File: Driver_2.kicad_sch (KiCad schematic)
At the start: 34 parts

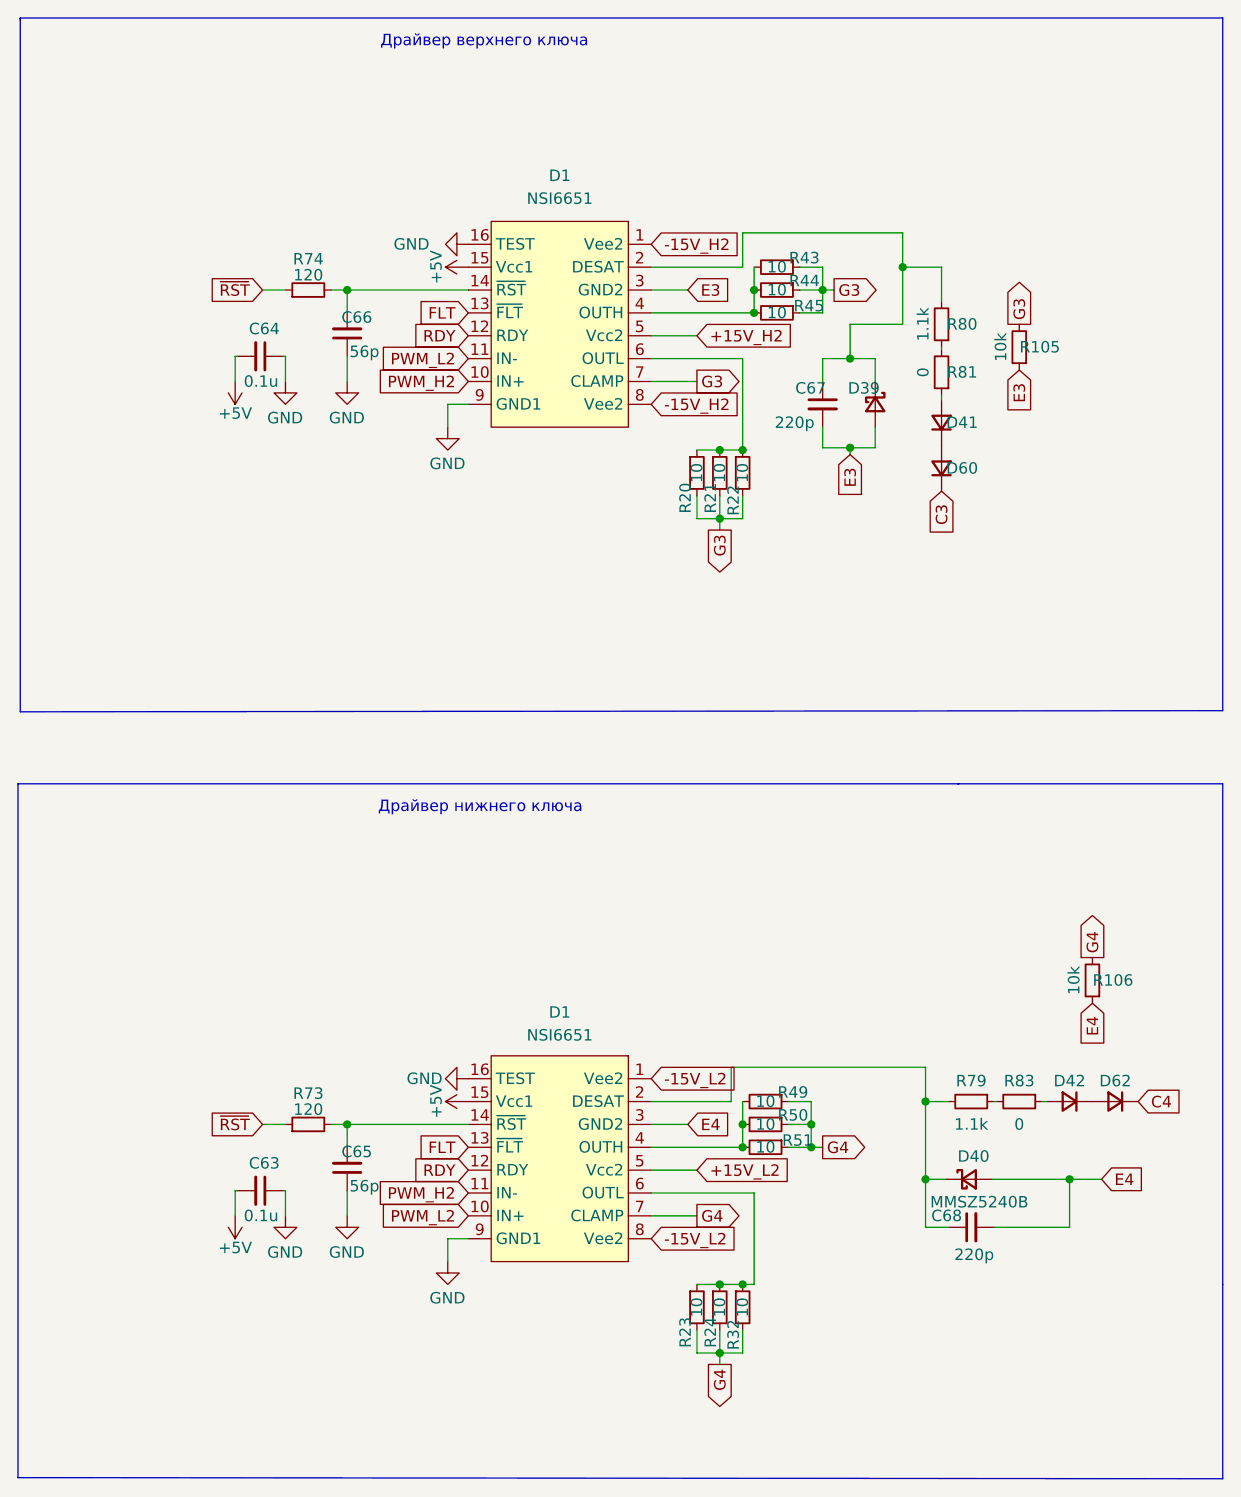
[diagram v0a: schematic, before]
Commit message: Развел вторую стойку
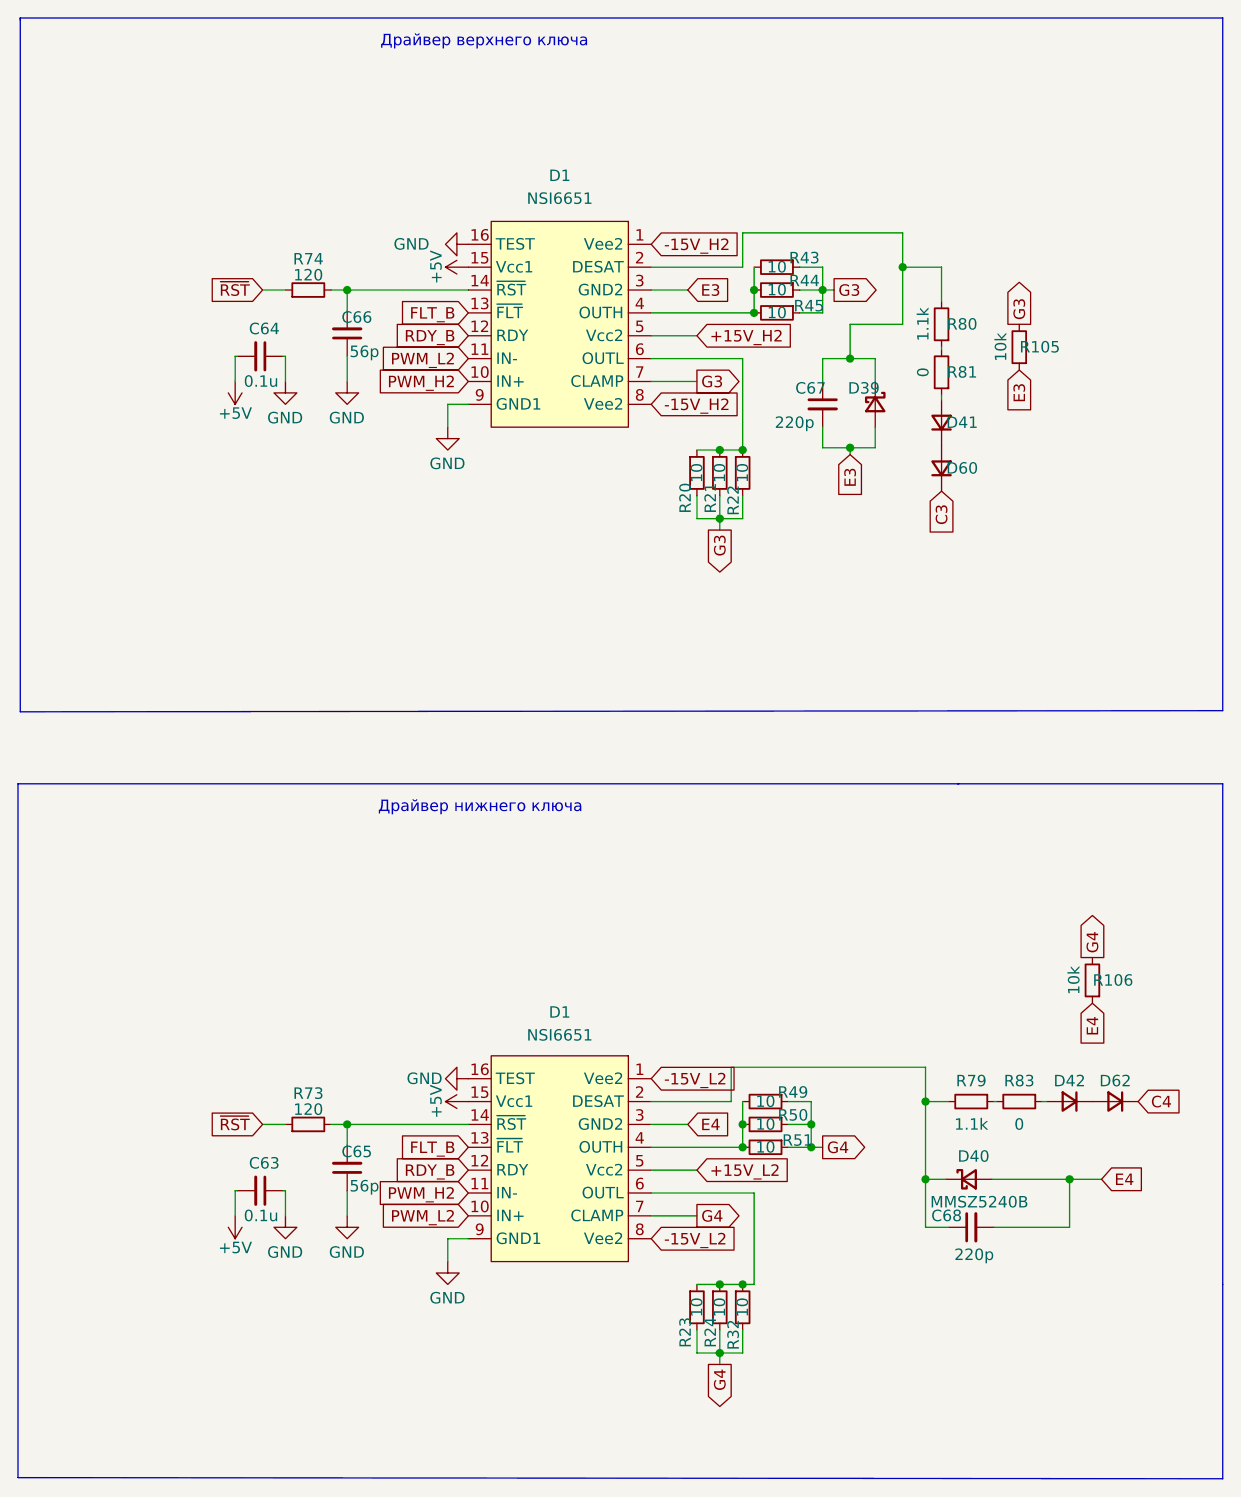
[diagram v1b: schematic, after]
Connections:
- net FLT renamed FLT_B
- net RDY renamed RDY_B
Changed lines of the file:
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@@
 		)
 	)
-	(global_label "FLT"
+	(global_label "FLT_B"
 		(shape input)
 		(at 81.28 55.88 180)
@@
 		)
 		(property "Intersheetrefs" "${INTERSHEET_REFS}"
-			(at 75.7206 55.88 0)
+			(at 72.9729 55.88 0)
 			(effects
 				(font
@@
 		)
 	)
-	(global_label "FLT"
+	(global_label "FLT_B"
 		(shape input)
 		(at 81.28 148.59 180)
@@
 		)
 		(property "Intersheetrefs" "${INTERSHEET_REFS}"
-			(at 75.7206 148.59 0)
+			(at 72.9729 148.59 0)
 			(effects
 				(font
@@
 		)
 	)
-	(global_label "RDY"
+	(global_label "RDY_B"
 		(shape input)
 		(at 81.28 58.42 180)
@@
 		)
 		(property "Intersheetrefs" "${INTERSHEET_REFS}"
-			(at 75.3384 58.42 0)
-			(effects
-				(font
-					(size 1.27 1.27)
-				)
-				(justify right)
-				(hide yes)
-			)
-		)
-	)
-	(global_label "RDY"
+			(at 72.4286 58.42 0)
+			(effects
+				(font
+					(size 1.27 1.27)
+				)
+				(justify right)
+				(hide yes)
+			)
+		)
+	)
+	(global_label "RDY_B"
 		(shape input)
 		(at 81.28 151.13 180)
@@
 		)
 		(property "Intersheetrefs" "${INTERSHEET_REFS}"
-			(at 75.3384 151.13 0)
-			(effects
-				(font
+			(at 72.4286 151.13 0)
+			(effects
+				(font
